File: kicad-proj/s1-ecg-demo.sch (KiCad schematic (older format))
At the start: 1 part

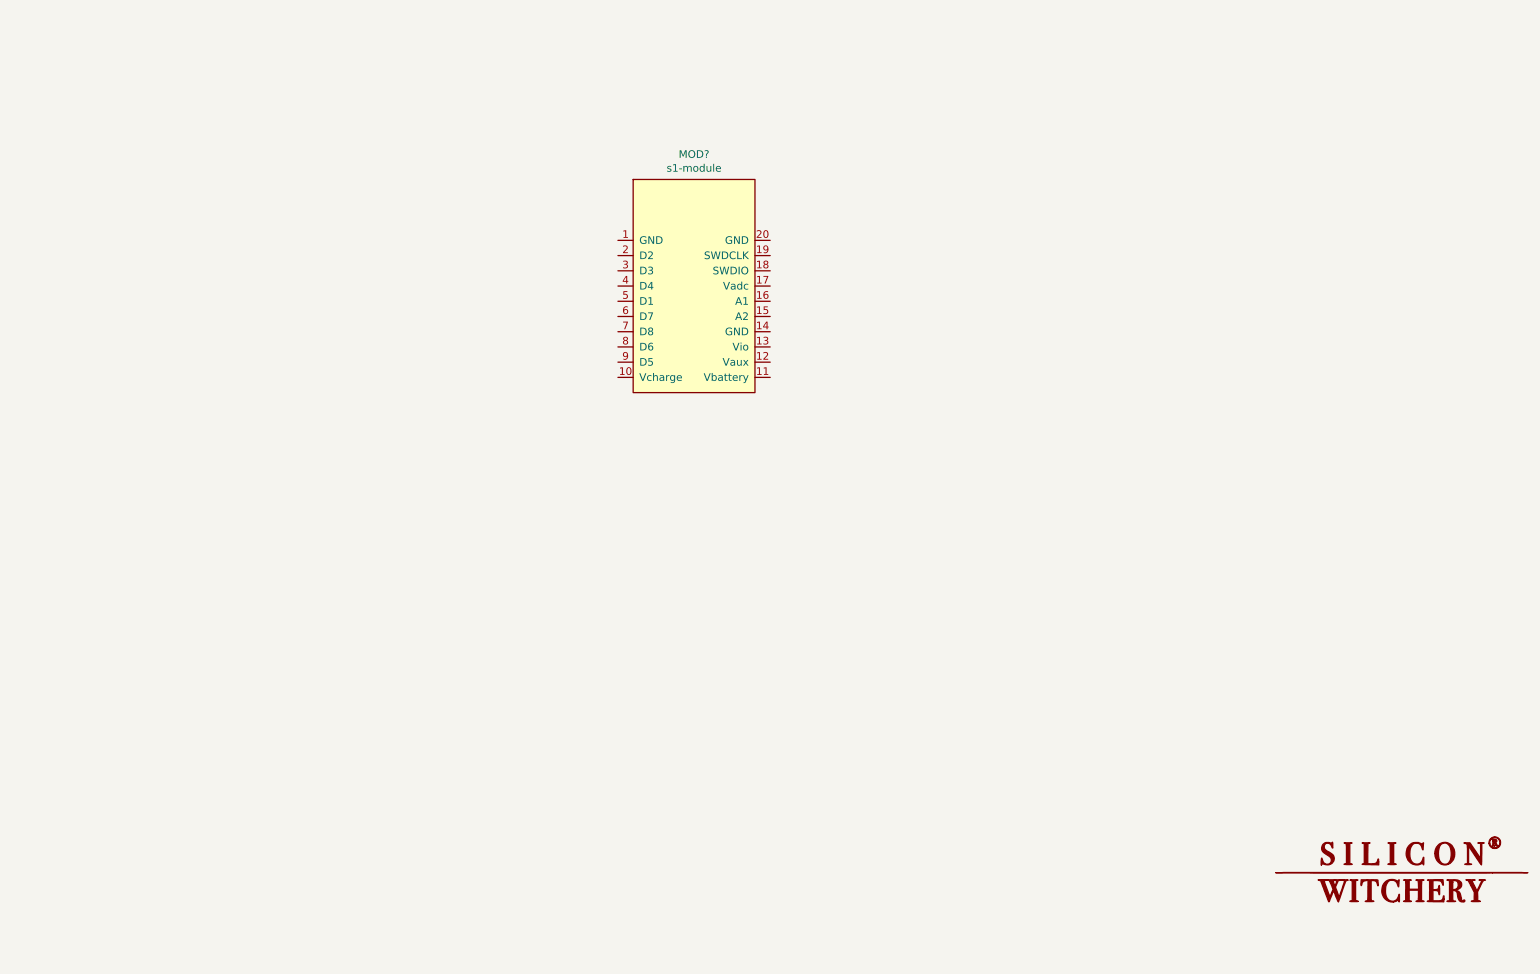
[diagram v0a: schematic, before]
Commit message: added schematic
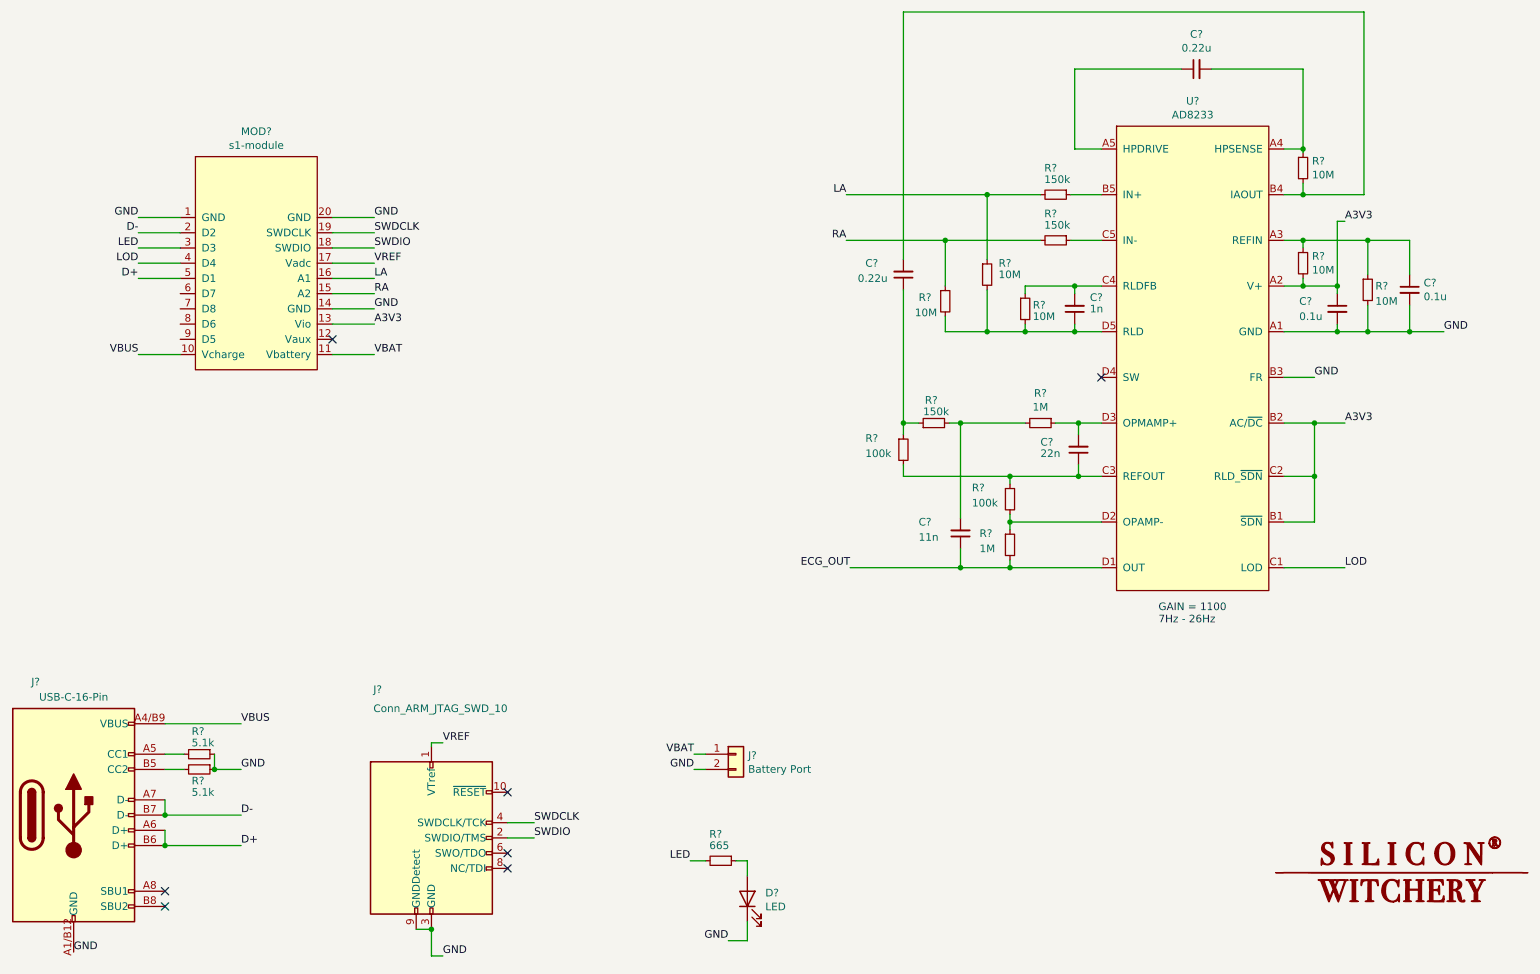
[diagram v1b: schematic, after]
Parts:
- added C? (x2): 0.22u, symbol Device:C_Small
- added C? (x2): 0.1u, symbol Device:C_Small
- added C?: 1n, symbol Device:C_Small
- added C?: 22n, symbol Device:C_Small
- added C?: 11n, symbol Device:C_Small
- added D?: LED, symbol Device:LED
- added J?: USB-C-16-Pin, symbol s1-ecg-demo:USB-C-16-Pin
- added J?: Conn_ARM_JTAG_SWD_10, symbol Connector:Conn_ARM_JTAG_SWD_10
- added J?: Battery Port, symbol Connector_Generic:Conn_01x02
- added R? (x2): 5.1k, symbol Device:R_Small
- added R? (x2): 1M, symbol Device:R_Small
- added R? (x2): 100k, symbol Device:R_Small
- added R? (x6): 10M, symbol Device:R_Small
- added R? (x3): 150k, symbol Device:R_Small
- added R?: 665, symbol Device:R_Small
- added U?: AD8233, symbol s1-ecg-demo:AD8233
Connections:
- net GND: now reaches MOD?.1 (GND)
- net GND: now also MOD?.14 (GND), MOD?.20 (GND), C?.2, C?.2, D?.1 (K), J?.2 (Pin_2), J?.3 (GND), J?.5 (GND), J?.9 (GNDDetect), J?.A1/B12 (GND), J?.A12/B1 (GND), R?.1, R?.1, R?.2, U?.A1 (GND), U?.B3 (FR)
- net VBUS: now reaches MOD?.10 (Vcharge)
- net VBUS: now also J?.A4/B9 (VBUS), J?.A9/B4 (VBUS)
- net VBAT: now reaches MOD?.11 (Vbattery)
- net VBAT: now also J?.1 (Pin_1)
- net A3V3: now reaches MOD?.13 (Vio)
- net A3V3: now also C?.1, R?.2, U?.A2 (V+), U?.B1 (~SDN), U?.B2 (AC/~DC), U?.C2 (RLD_~SDN)
- net RA: now reaches MOD?.15 (A2)
- net RA: now also R?.1, R?.2
- net LA: now reaches MOD?.16 (A1)
- net LA: now also R?.1, R?.2
- net VREF: now reaches MOD?.17 (Vadc)
- net VREF: now also J?.1 (VTref)
- net SWDIO: now reaches MOD?.18 (SWDIO)
- net SWDIO: now also J?.2 (SWDIO/TMS)
- net SWDCLK: now reaches MOD?.19 (SWDCLK)
- net SWDCLK: now also J?.4 (SWDCLK/TCK)
- net D-: now reaches MOD?.2 (D2)
- net D-: now also J?.A7 (D-), J?.B7 (D-)
- net LED: now reaches MOD?.3 (D3)
- net LED: now also R?.2
- net LOD: now reaches MOD?.4 (D4)
- net LOD: now also U?.C1 (LOD)
- net D+: now reaches MOD?.5 (D1)
- net D+: now also J?.A6 (D+), J?.B6 (D+)
- new net: C?.1, R?.1, R?.1, U?.A3 (REFIN)
- new net: C?.2, R?.1, U?.A4 (HPSENSE)
- new net: C?.1, U?.A5 (HPDRIVE)
- new net: C?.2, R?.2, U?.B4 (IAOUT)
- new net: R?.1, U?.B5 (IN+)
- new net: C?.1, R?.1, R?.2, U?.C3 (REFOUT)
- new net: C?.2, R?.1, U?.C4 (RLDFB)
- new net: R?.1, U?.C5 (IN-)
- new net: R?.1, R?.2, U?.D2 (OPAMP-)
- new net: C?.2, R?.1, U?.D3 (OPMAMP+)
- new net: C?.1, R?.2, R?.2, R?.2, U?.D5 (RLD)
- new net: J?.A5 (CC1), R?.2
- new net: J?.B5 (CC2), R?.2
- new net: C?.1, R?.1, R?.1
- new net: C?.2, R?.2, R?.2
- new net: D?.2 (A), R?.1
- new net ECG_OUT: C?.1, R?.2, U?.D1 (OUT)
- no-connect marks 0 -> 7
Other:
- note added: "GAIN = 1100\n7Hz - 26Hz"
- moved on the sheet: MOD?
